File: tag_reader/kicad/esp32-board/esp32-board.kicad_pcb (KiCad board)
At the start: 2 copper layers, 70.5 x 54.6 mm, 9 parts, among them J1 Conn_01x08_Pin, J2 Conn_01x04_Pin, J3 Conn_01x06_Pin, J4 Conn_01x15_Socket, J5 Conn_01x15_Socket, J6 Conn_01x15_Pin, J7 Conn_01x15_Pin, J8 Conn_01x06_Pin

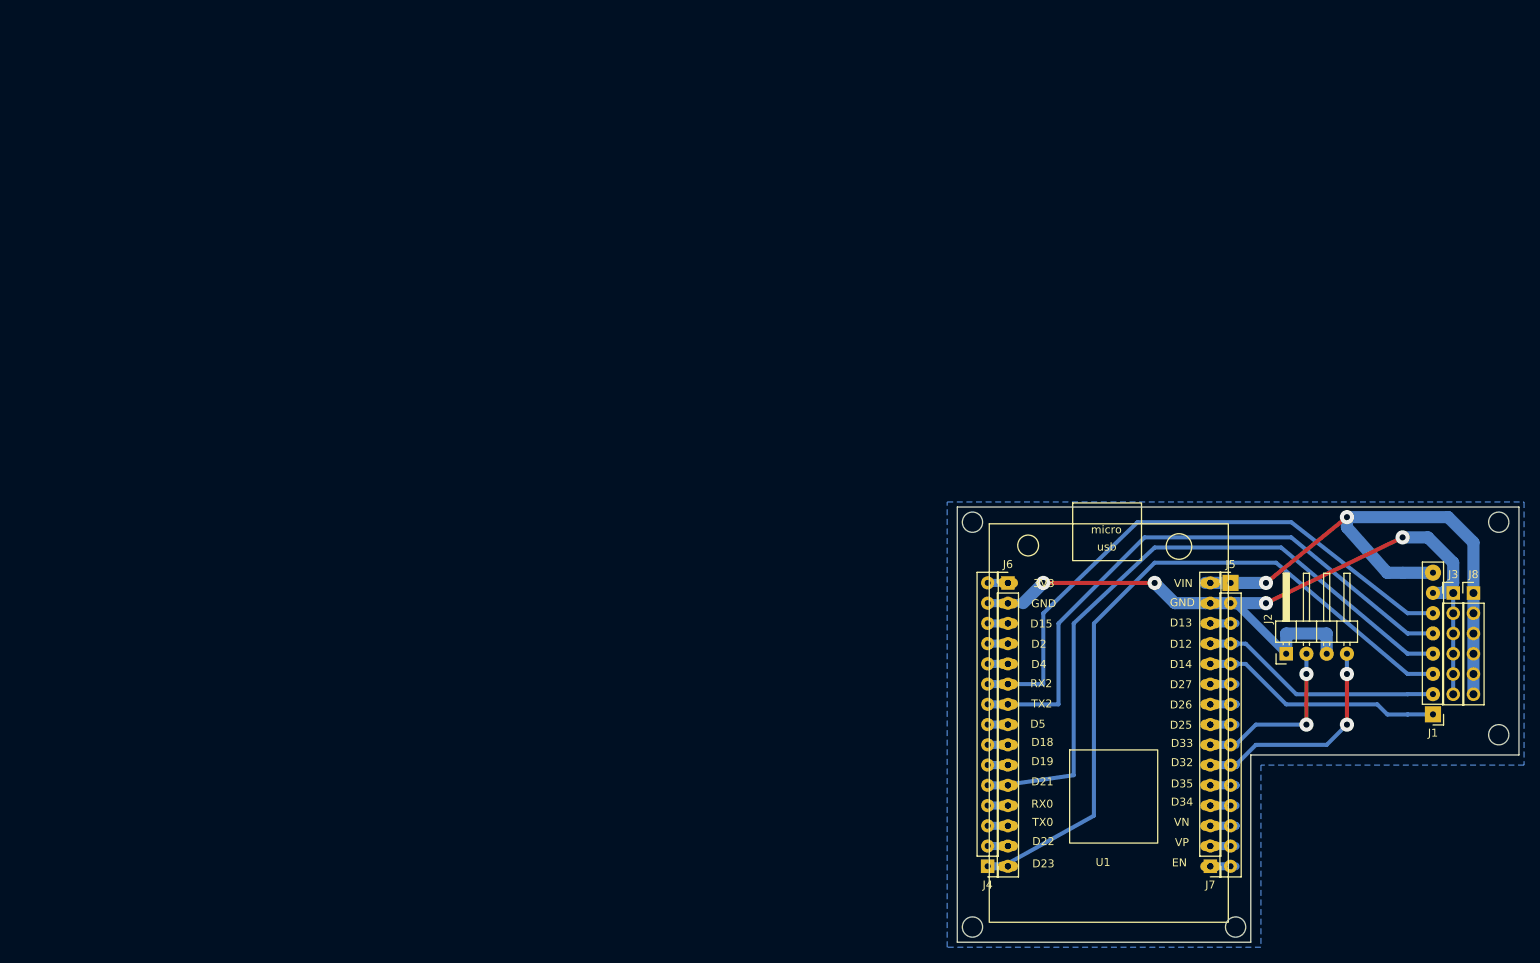
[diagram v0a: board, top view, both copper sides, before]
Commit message: making board
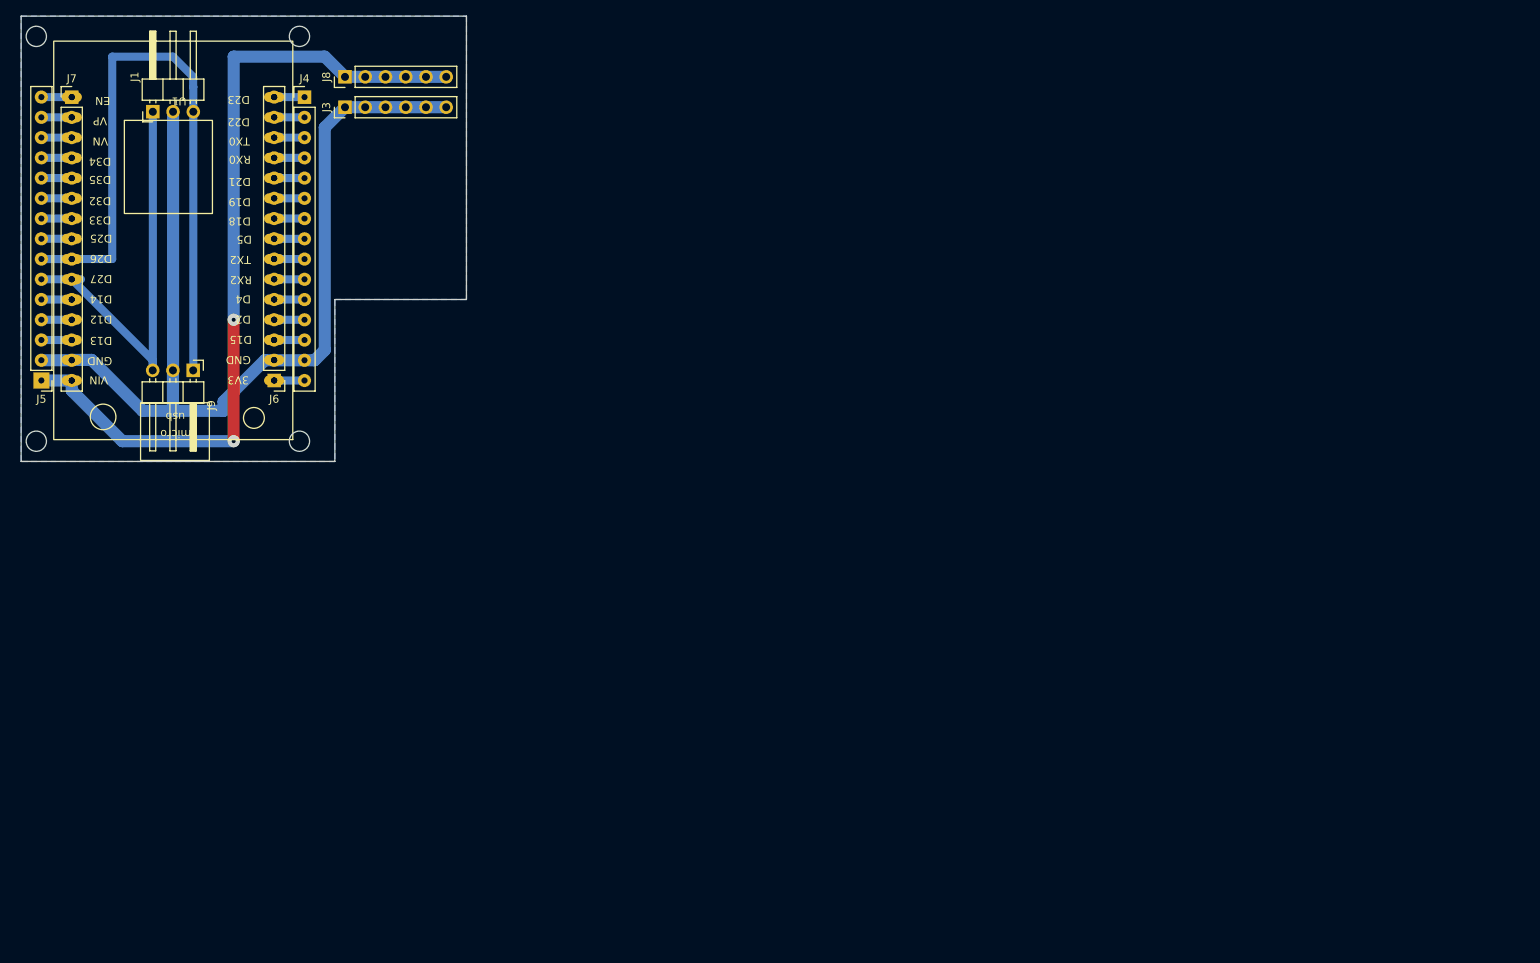
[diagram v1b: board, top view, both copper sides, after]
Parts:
- removed J2: Conn_01x04_Pin, Connector_PinHeader_2.54mm:PinHeader_1x04_P2.54mm_Horizontal
- added J9: Conn_01x03_Pin, Connector_PinHeader_2.54mm:PinHeader_1x03_P2.54mm_Horizontal, F.Cu at (22.2, 44.4)
- J1: value Conn_01x08_Pin -> Conn_01x03_Pin; footprint Connector_PinHeader_2.54mm:PinHeader_1x08_P2.54mm_Vertical -> Connector_PinHeader_2.54mm:PinHeader_1x03_P2.54mm_Horizontal
- moved J1 177.6 mm to (17.2, 12.0), turned to 90 degrees
- moved J7 172.4 mm to (6.98, 10.2), turned to 0 degrees
- moved J8 155.7 mm to (41.3, 7.62), turned to 90 degrees
- moved J3 151.8 mm to (41.3, 11.4), turned to 90 degrees
- moved J5 151.4 mm to (3.17, 45.7), turned to 180 degrees
- moved J4 129.1 mm to (36.2, 10.2), turned to 0 degrees
- moved U1 117.9 mm to (22.2, 40.6), turned to 180 degrees
- moved J6 95.5 mm to (32.4, 45.7), turned to 180 degrees
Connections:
- J1 pad 1: Net-(J1-Pin_1) -> D27
- J1 pad 2: Net-(J1-Pin_2) -> GND
- J1 pad 3: Net-(J1-Pin_3) -> D26
- J4 pad 1: Net-(J1-Pin_3) -> Net-(J4-Pin_1)
- J4 pad 10: Net-(J1-Pin_6) -> Net-(J4-Pin_10)
- J4 pad 5: Net-(J1-Pin_4) -> Net-(J4-Pin_5)
- J4 pad 9: Net-(J1-Pin_5) -> Net-(J4-Pin_9)
- J5 pad 4: Net-(J1-Pin_2) -> Net-(J5-Pin_4)
- J5 pad 5: Net-(J1-Pin_1) -> Net-(J5-Pin_5)
- J5 pad 6: Net-(J5-Pin_6) -> D27
- J5 pad 7: Net-(J5-Pin_7) -> D26
- J6 pad 11: Net-(J1-Pin_4) -> Net-(J4-Pin_5)
- J6 pad 15: Net-(J1-Pin_3) -> Net-(J4-Pin_1)
- J6 pad 6: Net-(J1-Pin_6) -> Net-(J4-Pin_10)
- J6 pad 7: Net-(J1-Pin_5) -> Net-(J4-Pin_9)
- J7 pad 10: Net-(J5-Pin_6) -> D27
- J7 pad 11: Net-(J1-Pin_1) -> Net-(J5-Pin_5)
- J7 pad 12: Net-(J1-Pin_2) -> Net-(J5-Pin_4)
- J7 pad 9: Net-(J5-Pin_7) -> D26
- U1 pad 11: Net-(J1-Pin_4) -> Net-(J4-Pin_5)
- U1 pad 15: Net-(J1-Pin_3) -> Net-(J4-Pin_1)
- U1 pad 24: Net-(J5-Pin_7) -> D26
- U1 pad 25: Net-(J5-Pin_6) -> D27
- U1 pad 26: Net-(J1-Pin_1) -> Net-(J5-Pin_5)
- U1 pad 27: Net-(J1-Pin_2) -> Net-(J5-Pin_4)
- U1 pad 6: Net-(J1-Pin_6) -> Net-(J4-Pin_10)
- U1 pad 7: Net-(J1-Pin_5) -> Net-(J4-Pin_9)
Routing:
- net Net-(J1-Pin_3): track 90.6 -> 0.00 mm
- net Net-(J1-Pin_4): track 84.3 -> 0.00 mm
- net D26: track 0.00 -> 82.3 mm
- net Net-(J1-Pin_5): track 75.5 -> 0.00 mm
- net Net-(J1-Pin_6): track 74.0 -> 0.00 mm
- net D27: track 0.00 -> 53.1 mm
- net VCC: track 71.6 -> 104.0 mm
- net Net-(J1-Pin_2): track 31.2 -> 0.00 mm
- net Net-(J1-Pin_1): track 31.2 -> 0.00 mm
- net Net-(J5-Pin_10): track 28.8 -> 3.81 mm, vias 2 -> 0
- net GND: track 101.8 -> 123.8 mm, vias 4 -> 0
- net Net-(J5-Pin_9): track 22.6 -> 3.81 mm, vias 2 -> 0
- net Net-(J4-Pin_10): track 0.00 -> 3.81 mm
- net Net-(J4-Pin_1): track 0.00 -> 3.81 mm
- net Net-(J5-Pin_4): track 0.00 -> 3.81 mm
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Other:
- board size 70.5 x 54.6 mm -> 55.9 x 55.9 mm

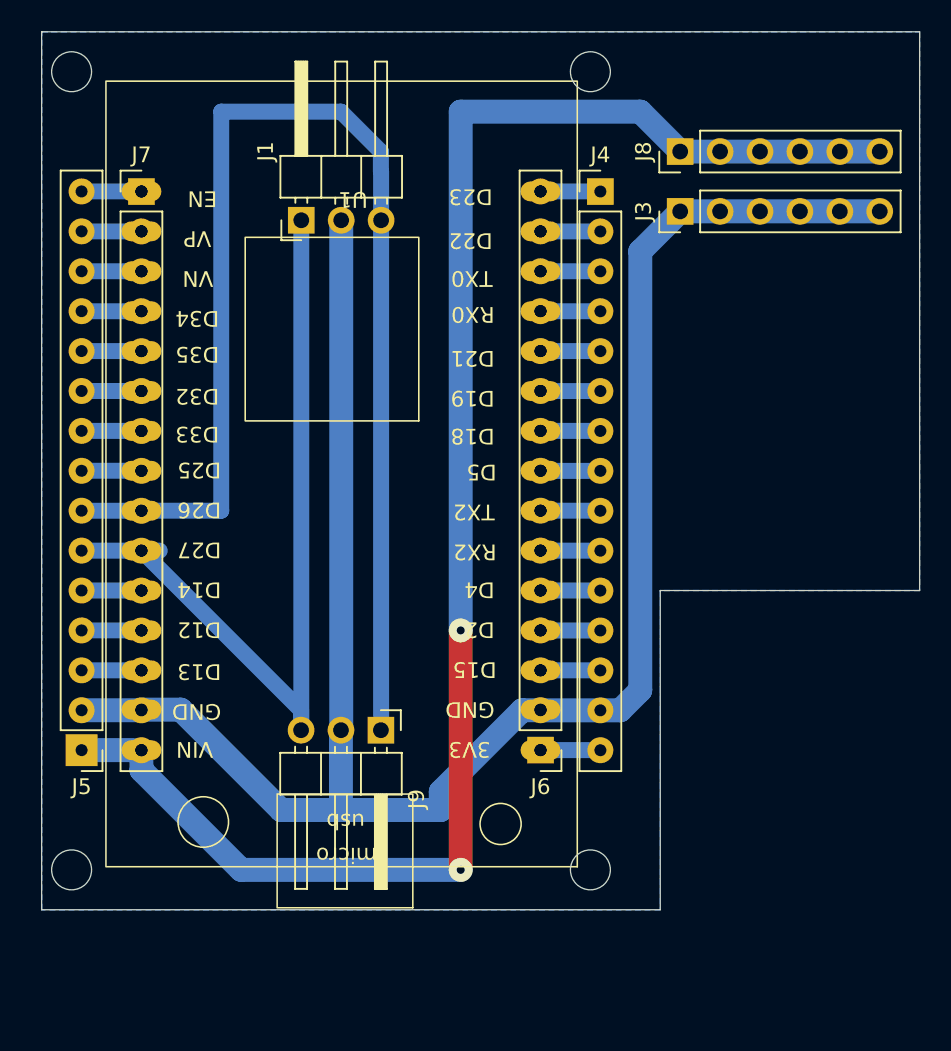
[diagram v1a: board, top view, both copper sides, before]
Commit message: compiling refactored, but not tested
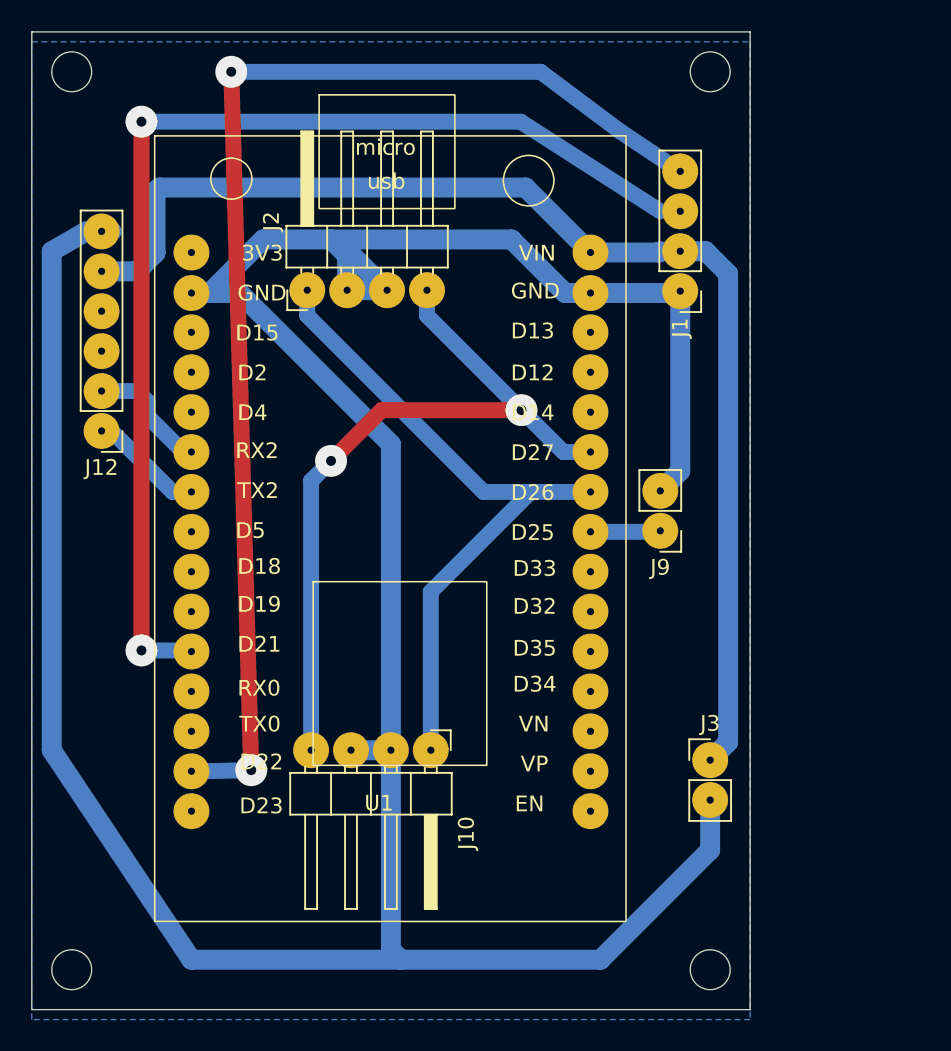
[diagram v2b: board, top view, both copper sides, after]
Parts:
- removed J4, J5: Conn_01x15_Socket, Connector_PinHeader_2.54mm:PinHeader_1x15_P2.54mm_Vertical
- removed J6, J7: Conn_01x15_Pin, Connector_PinHeader_2.54mm:PinHeader_1x15_P2.54mm_Vertical
- removed J8: Conn_01x06_Pin, Connector_PinHeader_2.54mm:PinHeader_1x06_P2.54mm_Vertical
- added J10: SW_LEFT, Connector_PinHeader_2.54mm:PinHeader_1x04_P2.54mm_Horizontal, F.Cu at (25.4, 45.7)
- added J12: LID, Connector_PinHeader_2.54mm:PinHeader_1x06_P2.54mm_Vertical, F.Cu at (4.45, 25.4)
- added J2: SW_RIGHT, Connector_PinHeader_2.54mm:PinHeader_1x04_P2.54mm_Horizontal, F.Cu at (17.5, 16.4)
- J1: value Conn_01x03_Pin -> OLED; footprint Connector_PinHeader_2.54mm:PinHeader_1x03_P2.54mm_Horizontal -> Connector_PinHeader_2.54mm:PinHeader_1x04_P2.54mm_Vertical
- J3: value Conn_01x06_Pin -> PWR; footprint Connector_PinHeader_2.54mm:PinHeader_1x06_P2.54mm_Vertical -> Connector_PinHeader_2.54mm:PinHeader_1x02_P2.54mm_Vertical
- J9: value Conn_01x03_Pin -> SPK; footprint Connector_PinHeader_2.54mm:PinHeader_1x03_P2.54mm_Horizontal -> Connector_PinHeader_2.54mm:PinHeader_1x02_P2.54mm_Vertical
- moved J3 35.0 mm to (43.2, 46.4), turned to 0 degrees
- moved J1 24.5 mm to (41.3, 16.5), turned to 180 degrees
- moved J9 21.8 mm to (40.0, 31.8), turned to 180 degrees
- moved U1 21.6 mm to (20.3, 19.1), turned to 0 degrees
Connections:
- J1 pad 1: D27 -> GND
- J1 pad 2: GND -> VCC
- J1 pad 3: D26 -> SCL
- J3 pad 1: GND -> VCC
- J9 pad 1: D26 -> SPK
- U1 pad 11: Net-(J4-Pin_5) -> SCL
- U1 pad 14: Net-(J4-Pin_2) -> SDA
- U1 pad 23: Net-(J5-Pin_8) -> SPK
- U1 pad 26: Net-(J5-Pin_5) -> LED1
- U1 pad 27: Net-(J5-Pin_4) -> LED2
- U1 pad 6: Net-(J4-Pin_10) -> RX2
- U1 pad 7: Net-(J4-Pin_9) -> TX2
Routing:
- net SDA: track 0.00 -> 79.4 mm, vias 0 -> 2
- net GND: track 123.8 -> 200.4 mm
- net SCL: track 0.00 -> 71.6 mm, vias 0 -> 2
- net D26: track 82.3 -> 43.4 mm
- net VCC: track 104.0 -> 76.4 mm, vias 2 -> 0
- net RX2: track 0.00 -> 7.23 mm
- net TX2: track 0.00 -> 6.69 mm
- net D27: track 53.1 -> 48.0 mm, vias 0 -> 2
- net SPK: track 0.00 -> 4.47 mm
- net Net-(J6-Pin_8): track 3.81 -> 0.00 mm
- net Net-(J6-Pin_5): track 3.81 -> 0.00 mm
- net Net-(J6-Pin_4): track 3.81 -> 0.00 mm
- net Net-(J6-Pin_3): track 3.81 -> 0.00 mm
- net Net-(J6-Pin_12): track 3.81 -> 0.00 mm
- net Net-(J4-Pin_10): track 3.81 -> 0.00 mm
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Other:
- board size 55.9 x 55.9 mm -> 45.7 x 62.2 mm
- board text added: "GND"
- board text added: "LED1"
- board text added: "LED2"
- board text added: "RX"
- board text added: "SCL"
- board text added: "SDA"
- board text added: "SPK"
- board text added: "TX"
- board text added: "VCC"
